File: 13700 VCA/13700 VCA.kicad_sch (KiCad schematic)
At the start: 47 parts, among them J101 Conn_02x05_Top_Bottom, J2 Conn_01x19, Q101 2N3906, Q102 2N3906, U101 LM13700, U102 TL072, U103 TL072

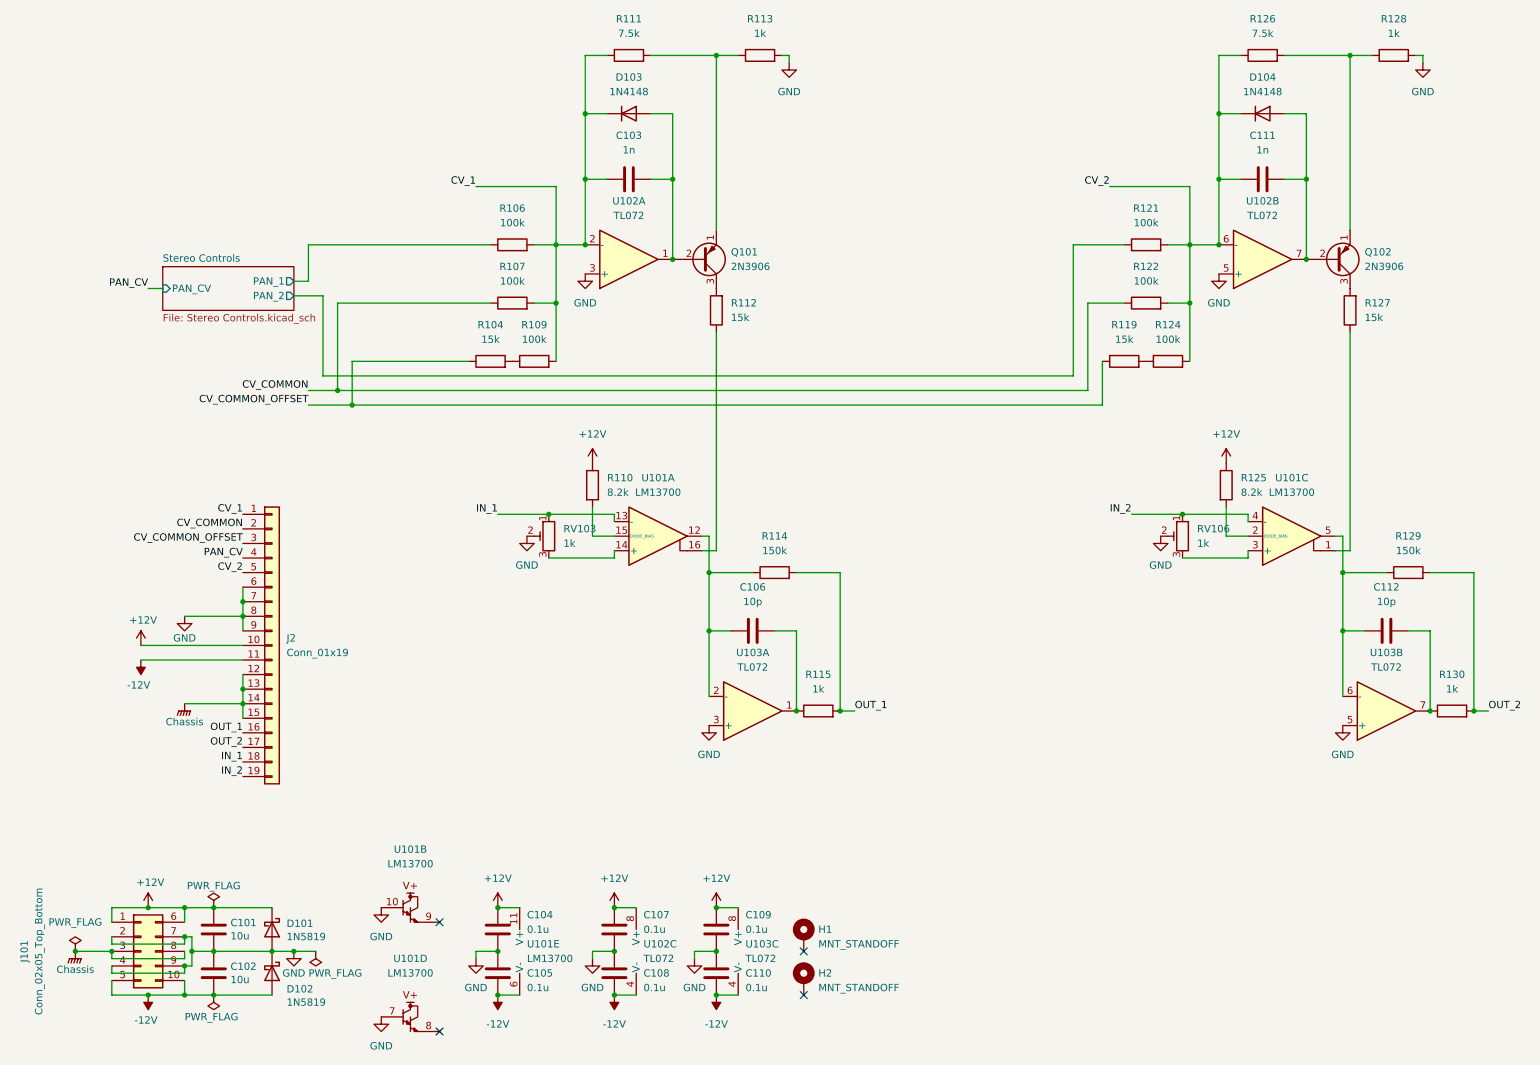
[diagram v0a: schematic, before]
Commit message: Begin revised delay
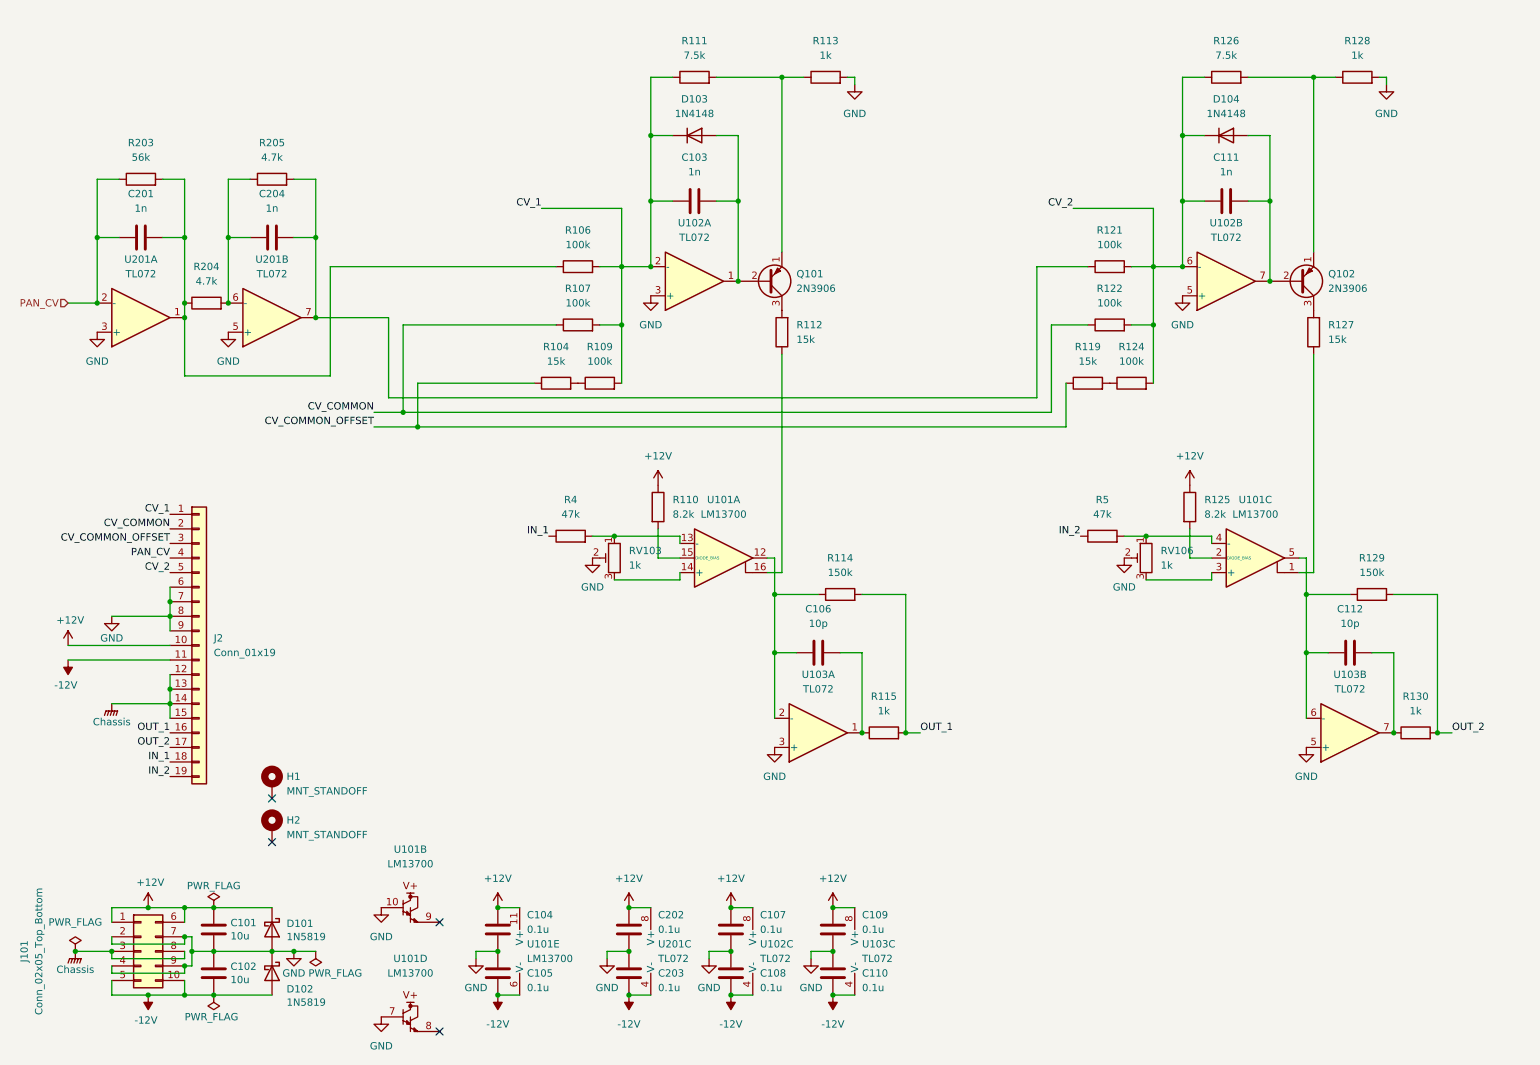
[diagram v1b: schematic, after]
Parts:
- added C201, C204: 1n, 0_Capacitor_THT:C_Disc_D5.5mm_W2.5mm_P2.50mm, symbol Device:C
- added C202, C203: 0.1u, 0_Capacitor_THT:C_Disc_D5.5mm_W2.5mm_P2.50mm, symbol Device:C
- added R203: 56k, Resistor_THT:R_Axial_DIN0207_L6.3mm_D2.5mm_P7.62mm_Horizontal, symbol Device:R
- added R204, R205: 4.7k, Resistor_THT:R_Axial_DIN0207_L6.3mm_D2.5mm_P7.62mm_Horizontal, symbol Device:R
- added R4, R5: 47k, Resistor_THT:R_Axial_DIN0207_L6.3mm_D2.5mm_P7.62mm_Horizontal, symbol Device:R
- added U201: TL072, Package_DIP:DIP-8_W7.62mm_Socket, symbol Amplifier_Operational:TL072
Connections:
- net +12V: now also C202.2, U201.8 (V+)
- net -12V: now also C203.1, U201.4 (V-)
- net GND: now also C202.1, C203.2, U201.3 (+), U201.5 (+)
- net IN_1: now also R4.1; no longer RV103.1, U101.13 (-)
- net IN_2: now also R5.1; no longer RV106.1, U101.4 (-)
- net PAN_CV: now also C201.1, R203.1, U201.2 (-)
- net Stereo Controls/PAN_1: no longer names the net of R106.1
- net Stereo Controls/PAN_1: now also C201.2, R203.2, R204.1, U201.1
- net Stereo Controls/PAN_2: no longer names the net of R121.1
- net Stereo Controls/PAN_2: now also C204.2, R205.2, U201.7
- new net: C204.1, R204.2, R205.1, U201.6 (-)
- new net: R5.2, RV106.1, U101.4 (-)
- new net: R4.2, RV103.1, U101.13 (-)
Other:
- removed sheet Stereo Controls
- moved on the sheet: C103, C106, C107, C108, C109, C110, C111, C112, D103, D104, H1, H2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
